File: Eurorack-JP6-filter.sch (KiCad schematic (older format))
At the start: 152 parts, among them J1 JACK_MONO_SW, J2 JACK_MONO_SW, J3 JACK_MONO_SW, J4 JACK_MONO_SW, J5 JACK_MONO_SW, J6 JACK_MONO_SW, P1 CONN_02X05, Q1 BCM857BS, Q2 BCM857BS, Q3 J112, Q4 J112, Q5 J112, Q6 J112, SW1 KS-01Q, U1 TL072-, U10 CD4027, U11 CD40106, U12 TS321, U13 TS321, U2 TL072-, U3 TL072-, U4 TL072-, U5 LM13700, U6 LM13700, U7 LM13700, U8 DG409, U9 CD4052

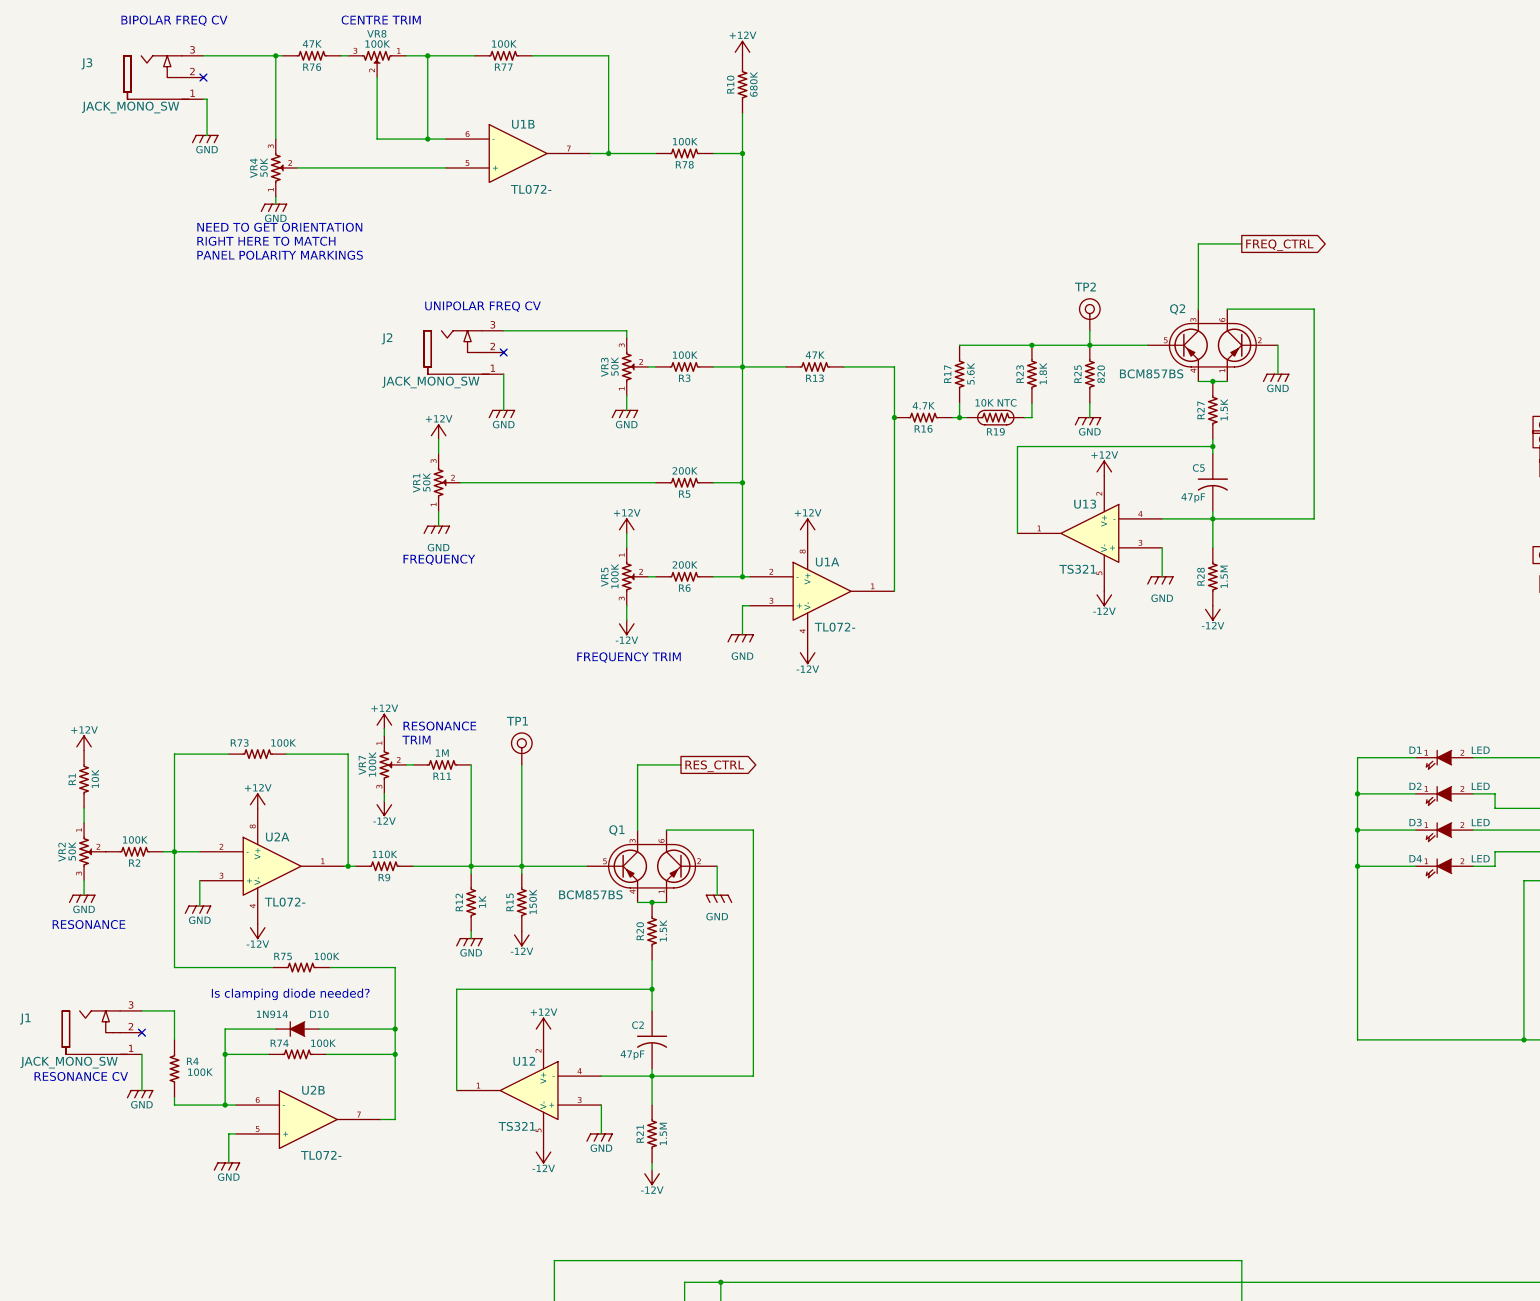
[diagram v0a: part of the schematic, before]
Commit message: hacking together v1.3 pcb
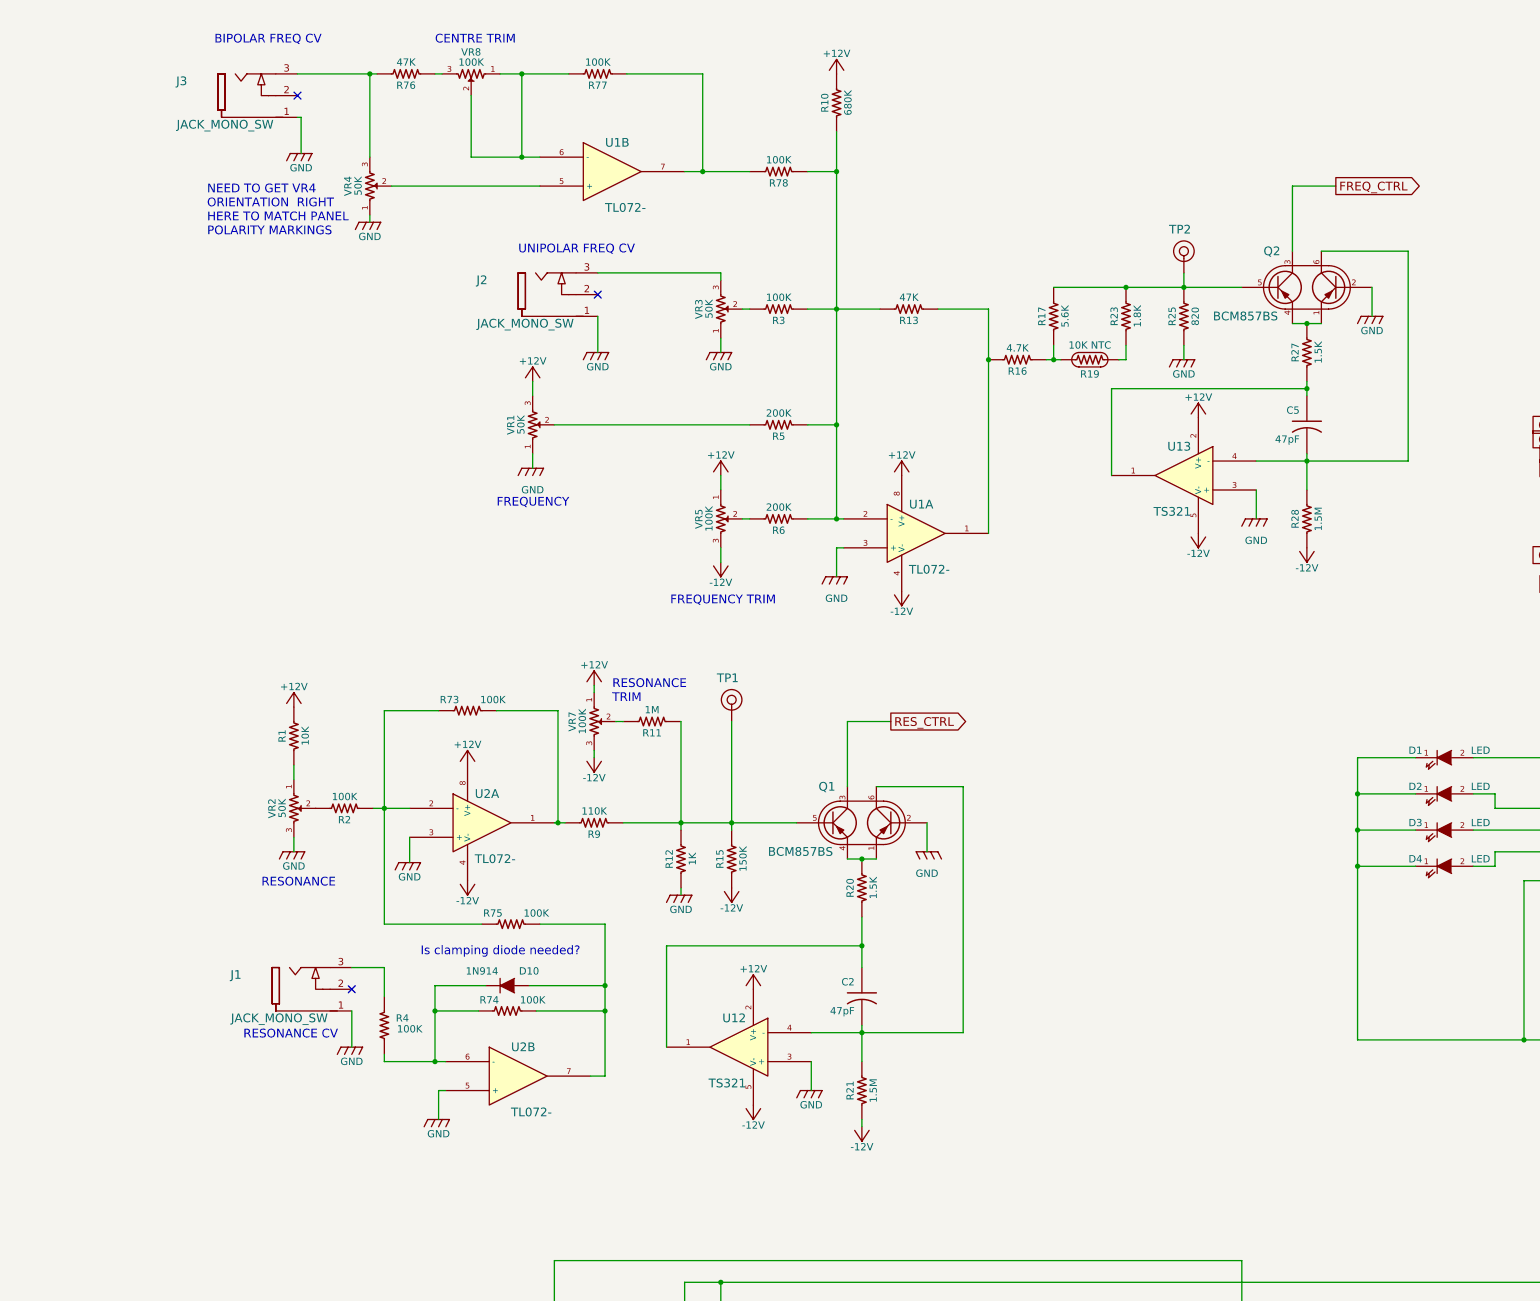
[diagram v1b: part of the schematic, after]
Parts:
- VR5, VR7: footprint MyModules:Bourns_3362P -> MyModules:TC33X-2
- VR8: footprint MyModules:RV16A-41-JRL -> MyModules:TC33X-2
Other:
- note added: "NEED TO GET VR4\nORIENTATION RIGHT\nHERE TO MATCH PANEL\nPOLARITY MARKINGS"
- note removed: "NEED TO GET ORIENTATION \nRIGHT HERE TO MATCH \nPANEL POLARITY MARKINGS"
- moved on the sheet: C2, C5, D10, J1, J2, J3, Q1, Q2, R1, R10, R11, R12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
